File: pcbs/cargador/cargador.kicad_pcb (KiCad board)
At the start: 2 copper layers, 57 x 58 mm, 38 parts, among them J1 Barrel_Jack, J2 Conn_01x04_Male, SW1 SW_SPST, U1 BQ24004, U2 LM2940-5V, U3 LM2575-3.3

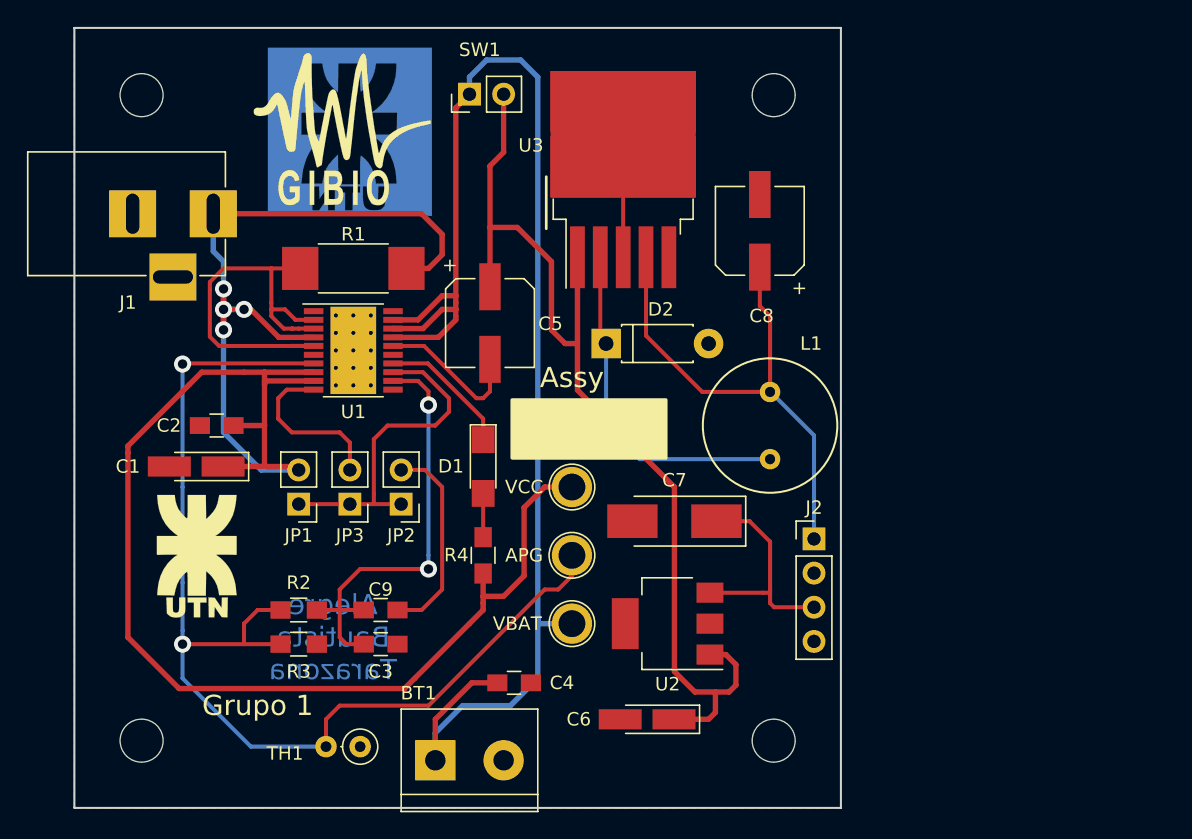
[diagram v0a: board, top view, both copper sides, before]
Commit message: pdfs realizados
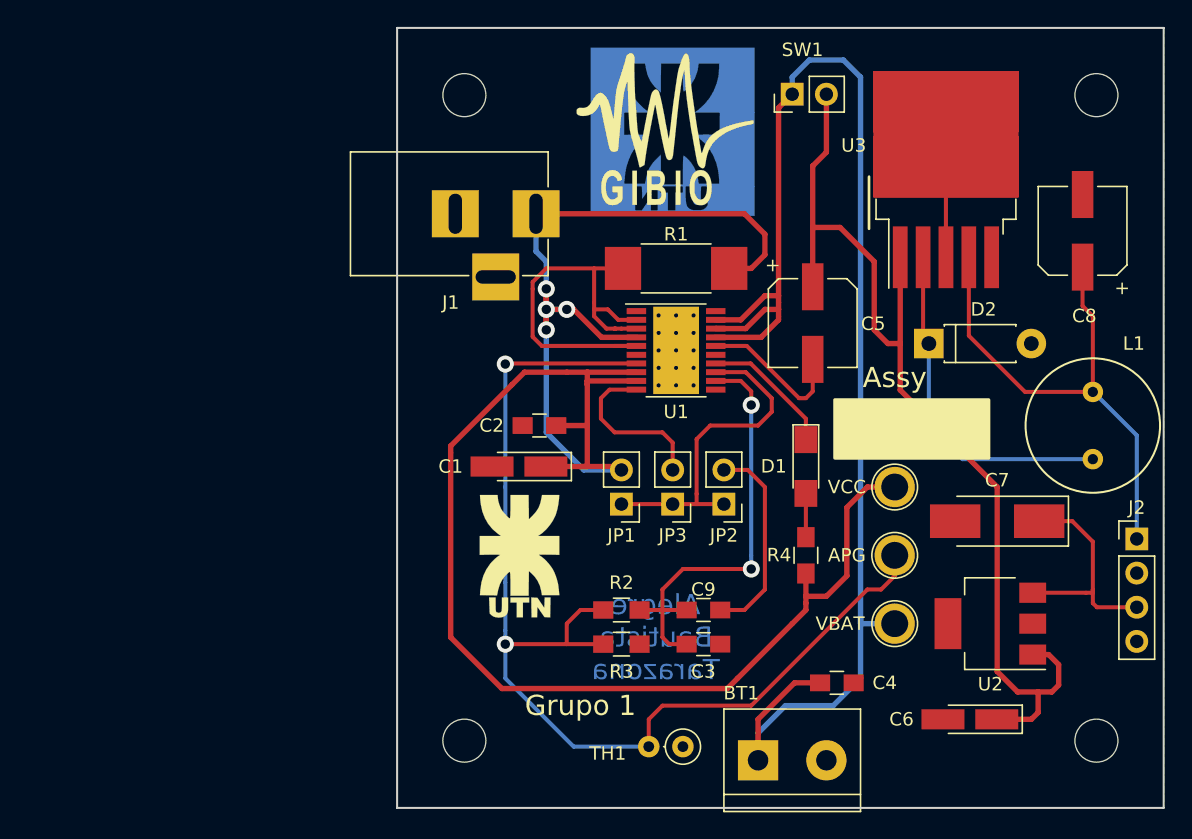
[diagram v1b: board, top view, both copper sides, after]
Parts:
- moved   24.0 mm to (134.5, 77.7)
- moved   24.0 mm to (133.7, 77.2)
- moved C3 24.0 mm to (136.8, 115.8)
- moved C9 24.0 mm to (136.8, 113.3)
- moved JP2 24.0 mm to (138.3, 105.4)
- moved JP3 24.0 mm to (134.5, 105.4)
- moved TH1 24.0 mm to (135.3, 123.4)
- moved    24.0 mm to (119.0, 123.0)
- moved    24.0 mm to (166.0, 75.0)
- moved   24.0 mm to (119.0, 75.0)
- moved   24.0 mm to (166.0, 123.0)
- moved   24.0 mm to (130.7, 83.3)
- moved   24.0 mm to (123.1, 109.0)
- moved APG 24.0 mm to (151.0, 109.2)
- moved BT1 24.0 mm to (140.8, 124.5)
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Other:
- board text added: "8.4V - 10V"
- board text added: "IMPORTANTE: - TH1: TERMISTOR: Resistors_THT:R_Axial_DIN0207_L6.3mm_D2.5mm_P2.54mm_Vertical. - R1: Resistors_SMD:R_2512_HandSoldering. - R2,R3 y R4 son 0805. - J1: BARREL JACK (o barrel jack cableado mejor para colocar en la caja. - C1: CP_Tantalum_Case-A_EIA-3216-18 - C2, C3 , C4 y C9 son 0805. - C5: CP_Elec_6.3x5.3. - C6: CP_Tantalum_Case-A_EIA-3216-18 - C7: CP_Tantalum_Case-C_EIA-6032-28 - C8: 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"
- board text added: "LLAVE ON/OFF"
- board text added: "MÓDULO CARGADOR DE BATERÍAS DE LI-ION"
- board text added: "PWR OUT"
- board text added: "VALORES: C1 = 10uF (Tantalio 3216) C2 = 0.1uF C3 = 0.22uF C4 = 1uF C5 = 100uF (Electrolítico) C6 = 0.47uF (Tantalio 3216) C7 = 47uF (Tantalio 6032) C8 = 330uF 50v (Electrolítico) C9 = 10pF D1 = LED 1206 D2 = 1N5817 L1 = 330uH CHOKE PK0810 R1 = 0.1 R R2 = 120 R R3 = 1K R4 = 470 R TH1 = 10K U1 = BQ24004. HTSSOP-20-1EP_4.4x6.5mm_Pitch0.65mm_ThermalPad U2 = LM2940 SOT-233-3pin (SMD) U3 = LM2575 TO-26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"
- board text added: "VBAT IN"
- board text added: "VIN"

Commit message: correcciones en los pdfs de los pcb
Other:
- board text added: "VALORES: C1 = 10uF (Tantalio 3216) C2 = 0.1uF C3 = 0.22uF C4 = 1uF C5 = 100uF (Electrolítico) C6 = 0.47uF (Tantalio 3216) C7 = 47uF (Tantalio 6032) C8 = 330uF 50v (Electrolítico) C9 = 10pF D1 = LED 1206 D2 = 1N5817 L1 = 330uH CHOKE PK0810 R1 = 0.1 R R2 = 120 R R3 = 1K R4 = 470 R TH1 = 10K, ANCHO PATA 0.7 o menos U1 = BQ24004. HTSSOP-20-1EP_4.4x6.5mm_Pitch0.65mm_ThermalPad U2 = LM2940 SOT-233-3pin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"
- board text removed: "VALORES: C1 = 10uF (Tantalio 3216) C2 = 0.1uF C3 = 0.22uF C4 = 1uF C5 = 100uF (Electrolítico) C6 = 0.47uF (Tantalio 3216) C7 = 47uF (Tantalio 6032) C8 = 330uF 50v (Electrolítico) C9 = 10pF D1 = LED 1206 D2 = 1N5817 L1 = 330uH CHOKE PK0810 R1 = 0.1 R R2 = 120 R R3 = 1K R4 = 470 R TH1 = 10K U1 = BQ24004. HTSSOP-20-1EP_4.4x6.5mm_Pitch0.65mm_ThermalPad U2 = LM2940 SOT-233-3pin (SMD) U3 = LM2575 TO-26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"
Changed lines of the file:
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@@
 (kicad_pcb (version 4) (host pcbnew 4.0.7-e2-6376~58~ubuntu16.04.1)
   (general
-    (links 69)
+    (links 0)
     (no_connects 0)
-    (area 30 37.525 279.285709 177.75)
+    (area 22.098 37.525 279.285709 189.136)
     (thickness 1.6)
     (drawings 36)
@@
   )
   (layers
-    (0 F.Cu signal hide)
-    (31 B.Cu signal hide)
+    (0 F.Cu signal)
+    (31 B.Cu signal)
     (32 B.Adhes user)
     (33 F.Adhes user)
@@
     (effects (font (size 3 3) (thickness 0.75)))
   )
-  (gr_text "VALORES:\nC1 = 10uF (Tantalio 3216)\nC2 = 0.1uF\nC3 = 0.22uF\nC4 = 1uF\nC5 = 100uF (Electrolítico)\nC6 = 0.47uF (Tantalio 3216)\nC7 = 47uF (Tantalio 6032)\nC8 = 330uF 50v (Electrolítico)\nC9 = 10pF\nD1 = LED 1206\nD2 = 1N5817\nL1 = 330uH CHOKE PK0810\nR1 = 0.1 R\nR2 = 120 R\nR3 = 1K\nR4 = 470 R\nTH1 = 10K\nU1 = BQ24004. HTSSOP-20-1EP_4.4x6.5mm_Pitch0.65mm_ThermalPad\nU2 = LM2940 SOT-233-3pin (SMD)\nU3 = LM2575 TO-263-5pin (SMD)" (at 197 96) (layer Cmts.User)
+  (gr_text "VALORES:\nC1 = 10uF (Tantalio 3216)\nC2 = 0.1uF\nC3 = 0.22uF\nC4 = 1uF\nC5 = 100uF (Electrolítico)\nC6 = 0.47uF (Tantalio 3216)\nC7 = 47uF (Tantalio 6032)\nC8 = 330uF 50v (Electrolítico)\nC9 = 10pF\nD1 = LED 1206\nD2 = 1N5817\nL1 = 330uH CHOKE PK0810\nR1 = 0.1 R\nR2 = 120 R\nR3 = 1K\nR4 = 470 R\nTH1 = 10K, ANCHO PATA 0.7 o menos\nU1 = BQ24004. HTSSOP-20-1EP_4.4x6.5mm_Pitch0.65mm_ThermalPad\nU2 = LM2940 SOT-233-3pin (SMD)\nU3 = LM2575 TO-263-5pin (SMD)" (at 197 96) (layer Cmts.User)
     (effects (font (size 1.5 1.5) (thickness 0.3)) (justify left))
   )
@@
     (arrow2b (pts (xy 169 133) (xy 167.873496 133.586421)))
   )
-  (gr_text "IMPORTANTE:\n- TH1: TERMISTOR: Resistors_THT:R_Axial_DIN0207_L6.3mm_D2.5mm_P2.54mm_Vertical.\n- R1: Resistors_SMD:R_2512_HandSoldering.\n- R2,R3 y R4 son 0805.\n- J1:  BARREL JACK (o barrel jack cableado mejor para colocar en la caja.\n- C1: CP_Tantalum_Case-A_EIA-3216-18\n- C2, C3 , C4 y C9 son 0805.\n- C5: CP_Elec_6.3x5.3.\n- C6: CP_Tantalum_Case-A_EIA-3216-18\n- C7: CP_Tantalum_Case-C_EIA-6032-28\n- C8: CP_Elec_6.3x7.7\n- D1: LED 1206. Tomando como referencia esta vista de la placa\n el ANODO(+) se conecta a la resistencia R4 y el CATODO(-) al bq24004.\n- D2: Diodes_THT:D_DO-41_SOD81_P7.62mm_Horizontal\n- L1: Choke_PK0810\n- U2: LM2940: SOT-223-3_TabPin2\n- U3: LM2575: TO-263-5_TabPin3" (at 30 156) (layer Cmts.User)
+  (gr_text "IMPORTANTE:\n- TH1: TERMISTOR: Resistors_THT:R_Axial_DIN0207_L6.3mm_D2.5mm_P2.54mm_Vertical.\n- R1: Resistors_SMD:R_2512_HandSoldering.\n- R2,R3 y R4 son 0805.\n- J1:  BARREL JACK (o barrel jack cableado mejor para colocar en la caja.\n- C1: CP_Tantalum_Case-A_EIA-3216-18\n- C2, C3 , C4 y C9 son 0805.\n- C5: CP_Elec_6.3x5.3.\n- C6: CP_Tantalum_Case-A_EIA-3216-18\n- C7: CP_Tantalum_Case-C_EIA-6032-28\n- C8: CP_Elec_6.3x7.7\n- D1: LED 1206. Tomando como referencia esta vista de la placa\n el ANODO(+) se conecta a la resistencia R4 y el CATODO(-) al bq24004.\n- D2: Diodes_THT:D_DO-41_SOD81_P7.62mm_Horizontal\n- L1: Choke_PK0810\n- U2: LM2940: SOT-223-3_TabPin2\n- U3: LM2575: TO-263-5_TabPin3" (at 22.098 167.386) (layer Cmts.User)
     (effects (font (size 1.5 1.5) (thickness 0.3)) (justify left))
   )
